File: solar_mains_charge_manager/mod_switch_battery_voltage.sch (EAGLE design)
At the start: 31 parts, among them IC1 ACS750LCA-050, T1 TIP122, X10 22-23-2041, X2 22-23-2021, X3 22-23-2031, X5 22-23-2031, X6 22-23-2041, X7 53047-15, X8 53047-15

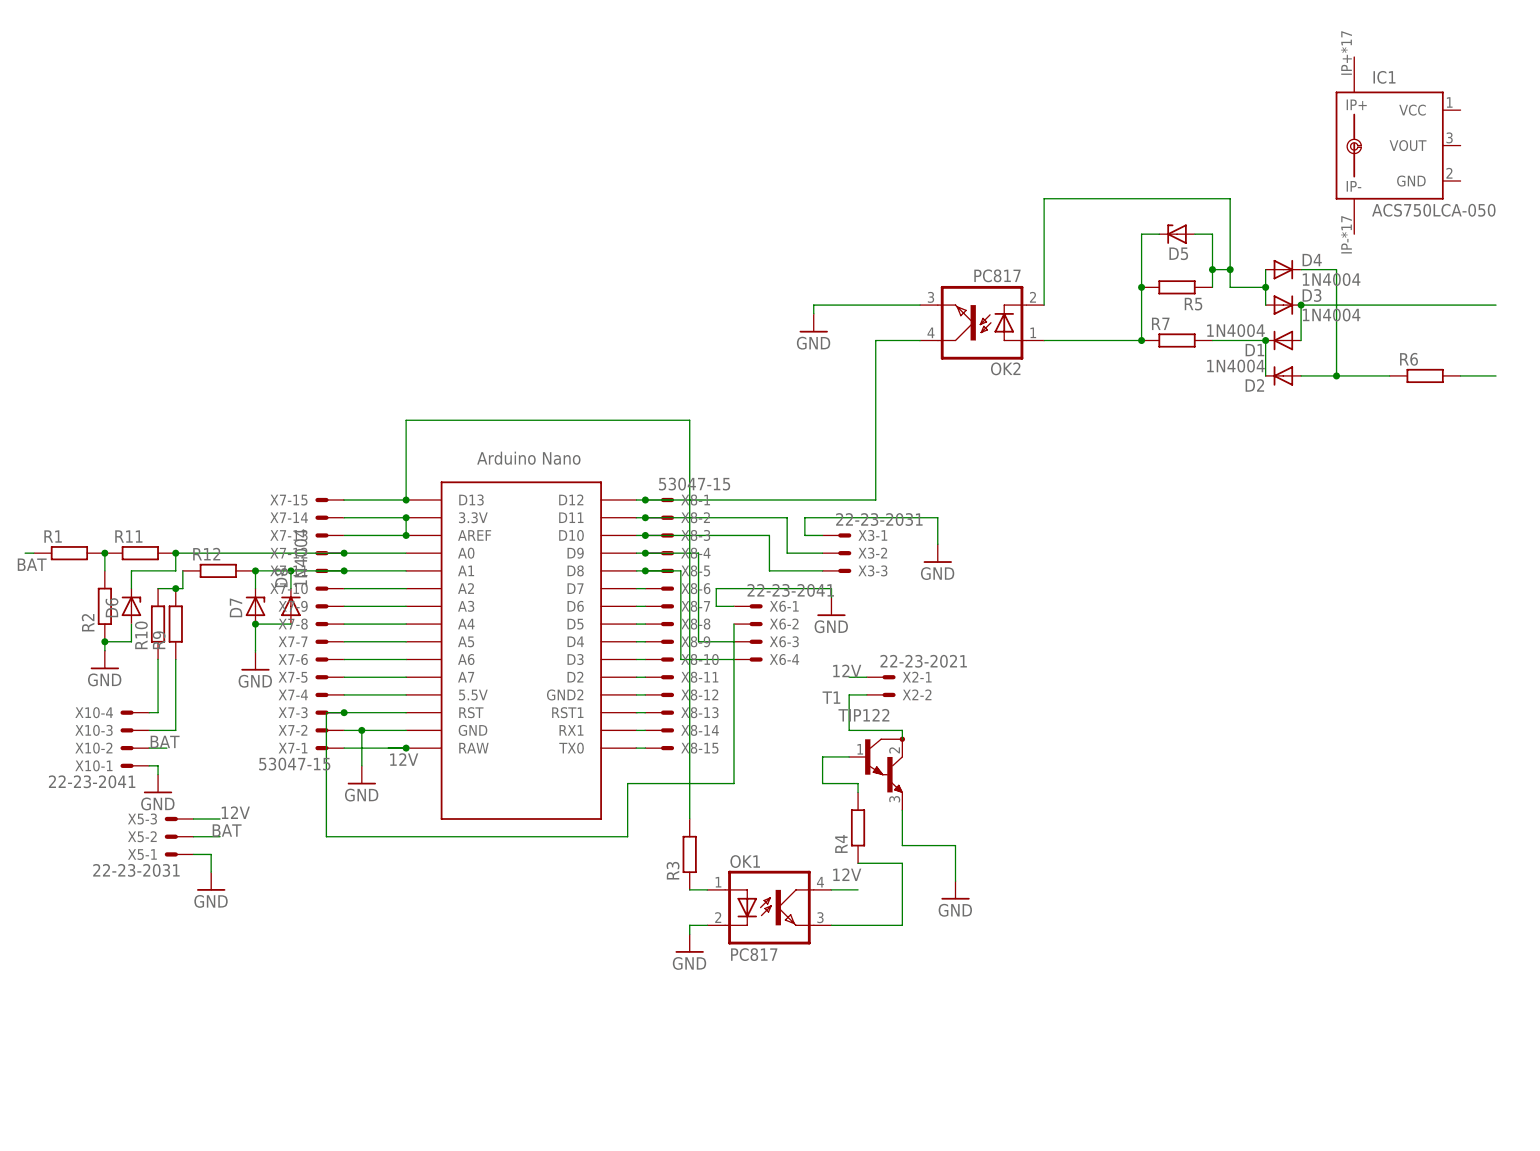
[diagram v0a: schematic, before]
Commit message: A lot of stuff
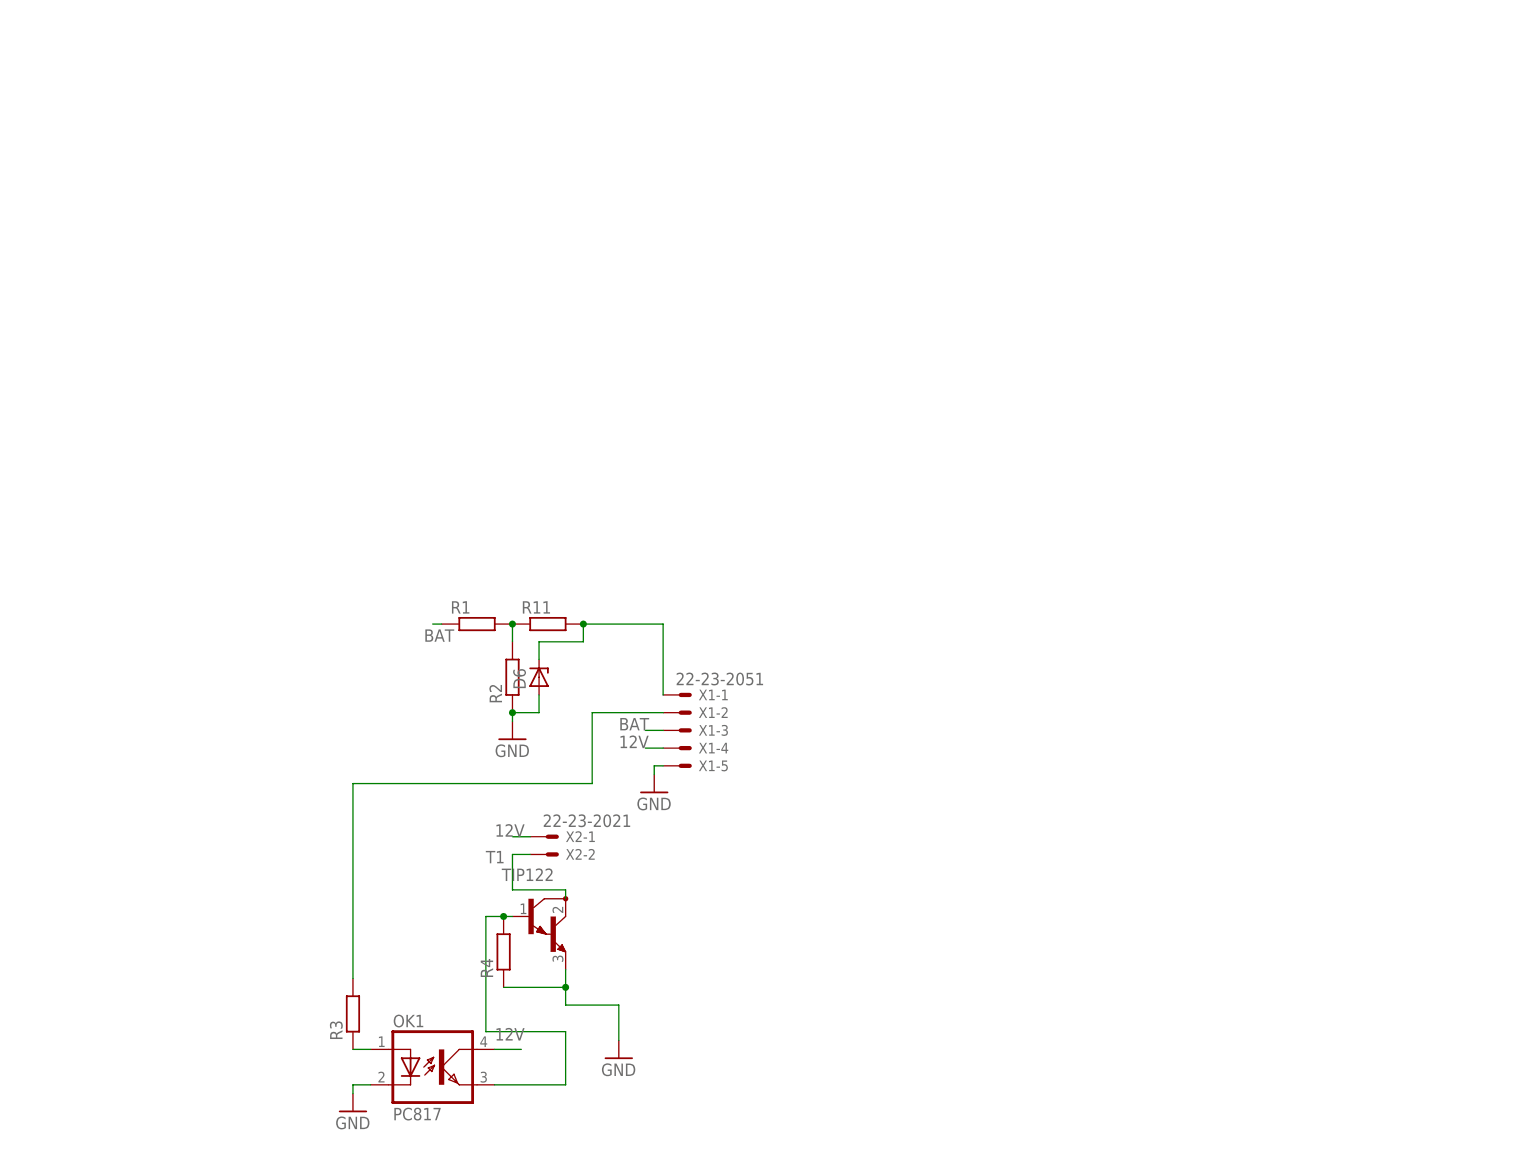
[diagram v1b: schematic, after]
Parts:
- removed D1, D2, D3, D4, D8: 1N4004, diode:1N4004
- removed D5, D7: (no value), diode:ZENER-DIODEDO34-7
- removed IC1: ACS750LCA-050, allegro:ACS750LCA-050
- removed OK2: PC817, optocoupler:PC817
- removed R10, R12, R5, R9: (no value), resistor:R-EU_0204/5
- removed R6, R7: (no value), resistor:R-EU_0204/7
- removed U$1: NANO, Arduino-clone:NANO
- removed X10, X6: 22-23-2041, con-molex:22-23-2041
- removed X3, X5: 22-23-2031, con-molex:22-23-2031
- removed X7, X8: 53047-15, con-molex:53047-15
- added X1: 22-23-2051, con-molex:22-23-2051
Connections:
- removed net N$1: U$1.3.3V, U$1.AREF, X7-13.S, X7-14.S
- removed net N$11: D1.C, D2.C, R7.2
- removed net N$12: OK2.COL, U$1.D12, X8-1.S
- removed net N$13: D1.A, D3.C
- removed net N$15: D2.A, D4.C, R6.1
- removed net N$16: R6.2
- removed net N$17: U$1.D11, X3-2.S, X8-2.S
- removed net N$18: U$1.D10, X3-3.S, X8-3.S
- removed net N$19: U$1.D9, X6-3.S, X8-4.S
- removed net N$2: R3.2, U$1.D13, X7-15.S
- removed net N$20: U$1.D8, X6-4.S, X8-5.S
- removed net N$21: U$1.RST, X6-2.S, X7-3.S
- removed net N$22: U$1.D7, X8-6.S
- removed net N$23: U$1.D6, X8-7.S
- removed net N$24: U$1.D5, X8-8.S
- removed net N$25: U$1.D4, X8-9.S
- removed net N$26: U$1.D3, X8-10.S
- removed net N$27: U$1.D2, X8-11.S
- removed net N$28: U$1.GND2, X8-12.S
- removed net N$29: U$1.RST1, X8-13.S
- removed net N$3: R10.2, R12.1, R9.2
- removed net N$30: U$1.RX1, X8-14.S
- removed net N$31: U$1.TX0, X8-15.S
- removed net N$32: U$1.5.5V, X7-4.S
- removed net N$33: U$1.A7, X7-5.S
- removed net N$34: U$1.A6, X7-6.S
- removed net N$35: U$1.A5, X7-7.S
- removed net N$36: U$1.A4, X7-8.S
- removed net N$37: U$1.A3, X7-9.S
- removed net N$38: U$1.A2, X7-10.S
- removed net N$39: D7.C, D8.C, R12.2, U$1.A1, X7-11.S
- removed net N$41: R10.1, X10-4.S
- removed net N$42: R9.1, X10-3.S
- removed net N$8: D3.A, D4.A, D5.A, OK2.C, R5.1
- removed net N$9: D5.C, OK2.A, R5.2, R7.1
- net 12V: now also X1-4.S; no longer U$1.RAW, X5-3.S, X7-1.S
- net BAT: now also X1-3.S; no longer X10-2.S, X5-2.S
- net GND: now also R4.1, X1-5.S; no longer D7.A, D8.A, OK2.EMIT, U$1.GND, X10-1.S, X3-1.S, X5-1.S, X6-1.S, X7-2.S
- net N$40: now also X1-1.S; no longer U$1.A0, X7-12.S
- net N$6: now also R3.2, X1-2.S; no longer OK1.EMIT, R4.1
- net N$7: now also OK1.EMIT
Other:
- moved on the sheet: D6, OK1, R1, R11, R2, R3, R4, T1, X2-1, X2-2
